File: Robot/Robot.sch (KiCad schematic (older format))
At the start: 2 parts

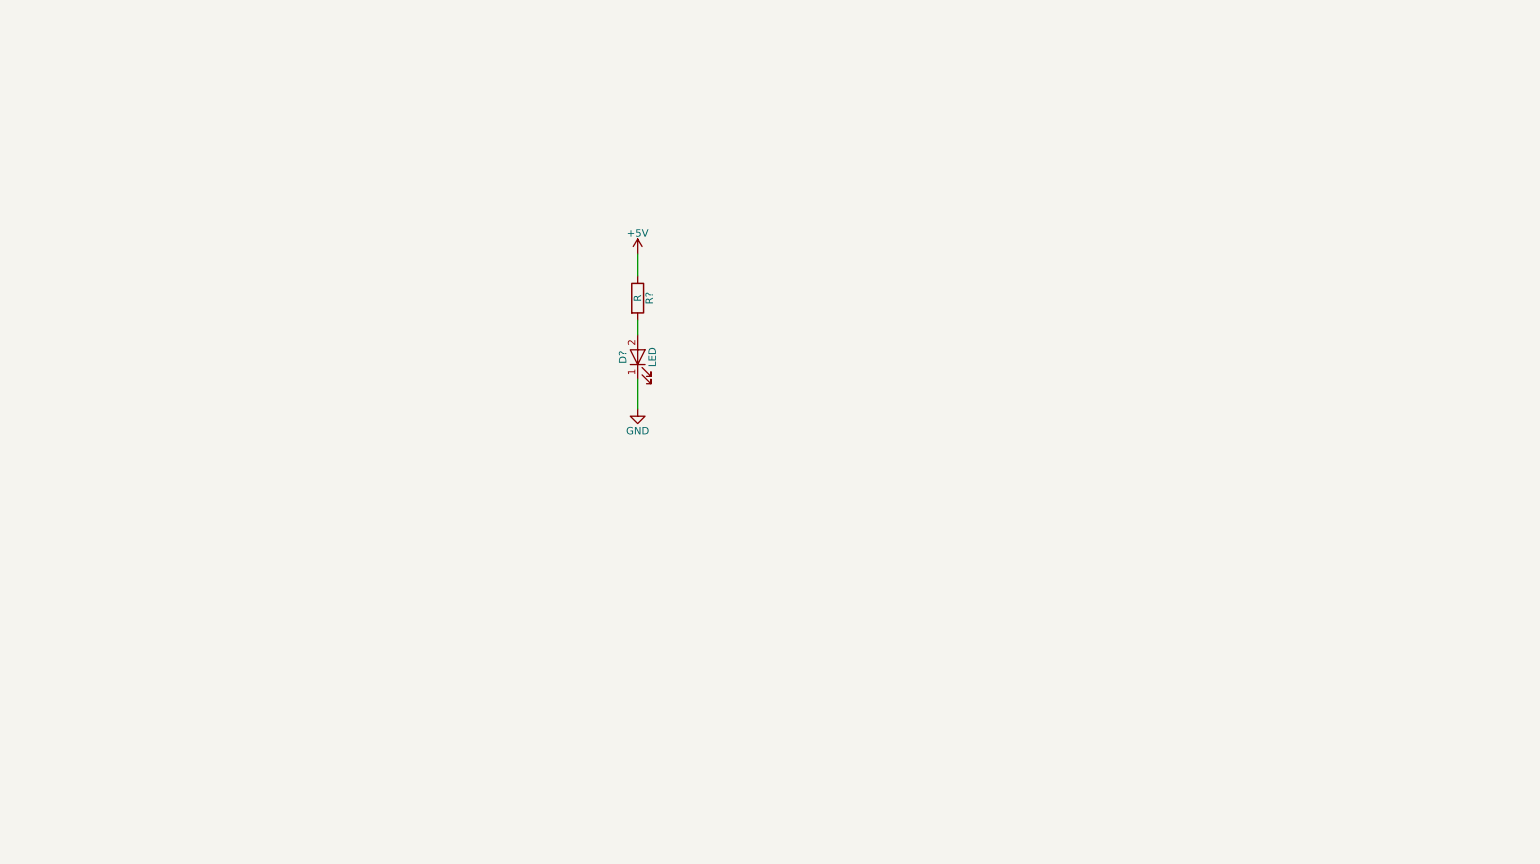
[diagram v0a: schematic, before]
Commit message: shema
shema
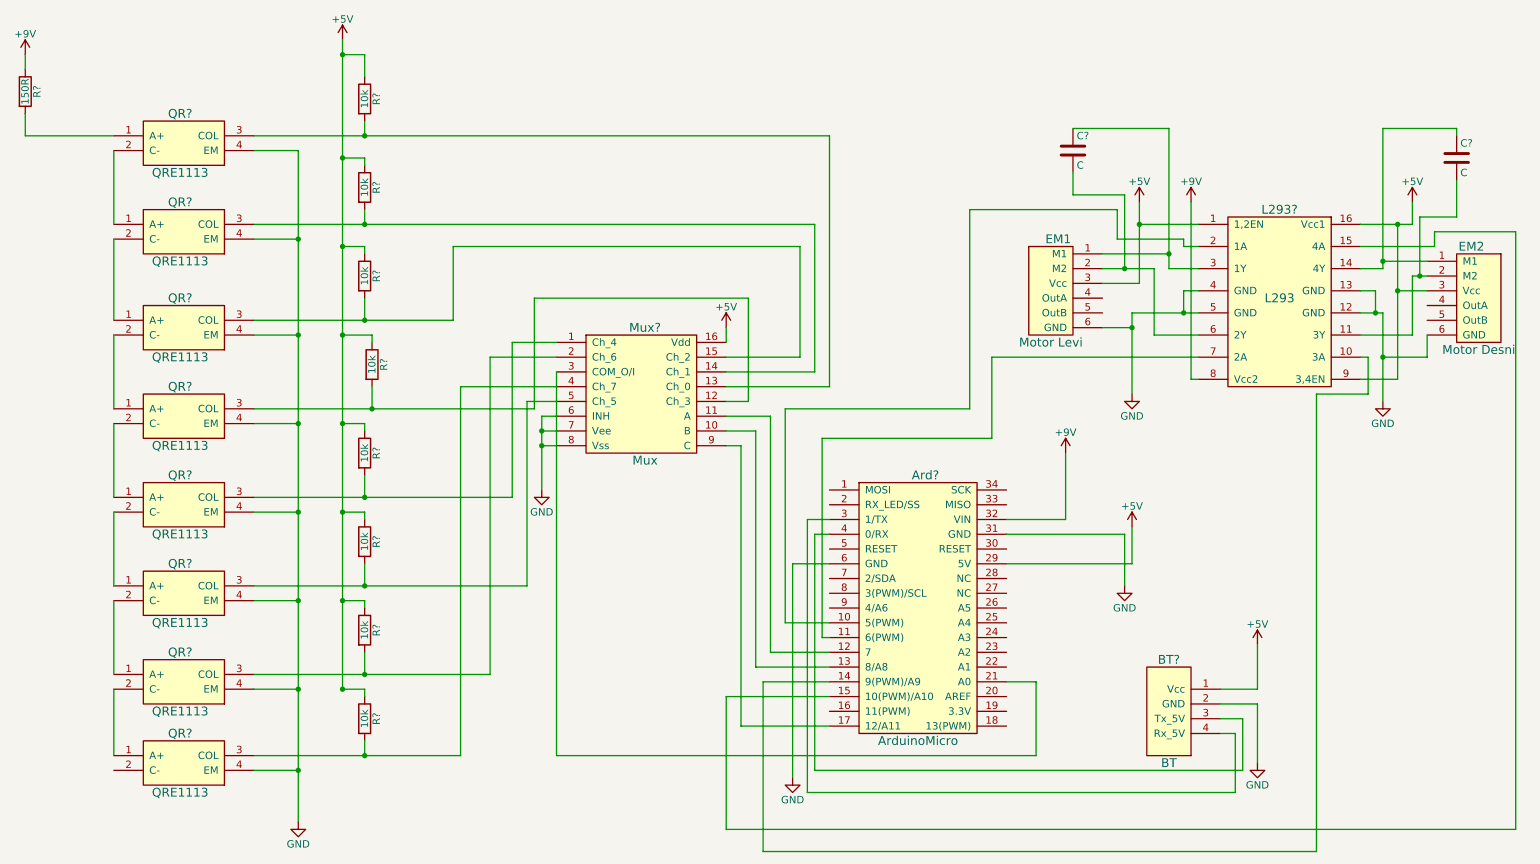
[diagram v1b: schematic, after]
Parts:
- removed D?: LED, symbol LED
- removed R?: R, symbol R
- added Ard?: ArduinoMicro, symbol ArduinoMicro
- added BT?: BT, symbol BT
- added C? (x2): C, symbol C
- added EM1: Motor Levi, symbol Motor
- added EM2: Motor Desni, symbol Motor
- added L293?: L293, symbol L293
- added Mux?: Mux, symbol Mux
- added QR? (x8): QRE1113, symbol QRE1113
- added R?: 150R, symbol R
- added R? (x8): 10k, symbol R
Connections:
- net +5V: now also Ard?.29 (5V), BT?.1 (Vcc), EM1.3 (Vcc), EM2.3 (Vcc), L293?.1 (1,2EN), L293?.16 (Vcc1), L293?.9 (3,4EN), Mux?.16 (Vdd), R?.1, R?.1, R?.1, R?.1, R?.1, R?.1, R?.1, R?.1
- net GND: now also Ard?.31 (GND), Ard?.6 (GND), BT?.2 (GND), EM1.6 (GND), EM2.6 (GND), L293?.12 (GND), L293?.13 (GND), L293?.4 (GND), L293?.5 (GND), Mux?.6 (INH), Mux?.7 (Vee), Mux?.8 (Vss), QR?.4 (EM), QR?.4 (EM), QR?.4 (EM), QR?.4 (EM), QR?.4 (EM), QR?.4 (EM), QR?.4 (EM), QR?.4 (EM)
- new net: QR?.1 (A+), R?.2
- new net: QR?.1 (A+), QR?.2 (C-) (x7)
- new net: Mux?.13 (Ch_0), QR?.3 (COL), R?.2
- new net: Ard?.14 (9(PWM)/A9), L293?.10 (3A)
- new net: C?.2, EM2.2 (M2), L293?.11 (3Y)
- new net: C?.1, EM2.1 (M1), L293?.14 (4Y)
- new net: Ard?.15 (10(PWM)/A10), L293?.15 (4A)
- new net: Ard?.10 (5(PWM)), L293?.2 (1A)
- new net: C?.1, EM1.1 (M1), L293?.3 (1Y)
- new net: C?.2, EM1.2 (M2), L293?.6 (2Y)
- new net: Ard?.11 (6(PWM)), L293?.7 (2A)
- new net: Mux?.1 (Ch_4), QR?.3 (COL), R?.2
- new net: Ard?.13 (8/A8), Mux?.10 (B)
- new net: Ard?.12 (7), Mux?.11 (A)
- new net: Mux?.12 (Ch_3), QR?.3 (COL), R?.2
- new net: Mux?.14 (Ch_1), QR?.3 (COL), R?.2
- new net: Mux?.15 (Ch_2), QR?.3 (COL), R?.2
- new net: Mux?.2 (Ch_6), QR?.3 (COL), R?.2
- new net: Ard?.21 (A0), Mux?.3 (COM_O/I)
- new net: Mux?.4 (Ch_7), QR?.3 (COL), R?.2
- new net: Mux?.5 (Ch_5), QR?.3 (COL), R?.2
- new net: Ard?.17 (12/A11), Mux?.9 (C)
- new net: Ard?.3 (1/TX), BT?.4 (Rx_5V)
- new net: Ard?.4 (0/RX), BT?.3 (Tx_5V)
- new net +9V: Ard?.32 (VIN), L293?.8 (Vcc2), R?.1
